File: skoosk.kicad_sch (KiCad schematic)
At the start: 90 parts, among them SW1 SW_Push, U1 ProMicro

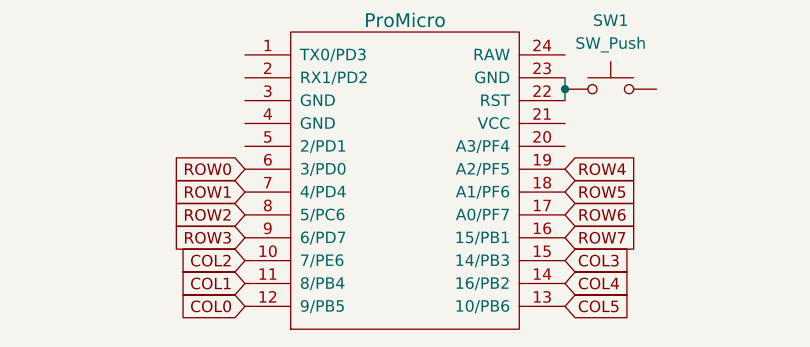
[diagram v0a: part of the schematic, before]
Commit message: saving before doing autorouting
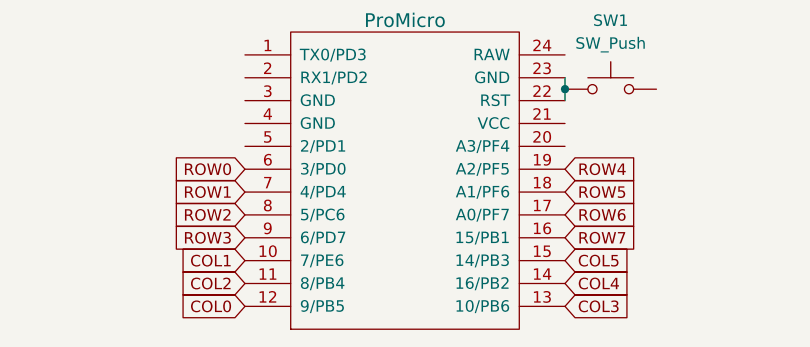
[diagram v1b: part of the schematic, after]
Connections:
- net COL1: now also U1.10 (7/PE6); no longer U1.11 (8/PB4)
- net COL2: now also U1.11 (8/PB4); no longer U1.10 (7/PE6)
- net COL3: now also U1.13 (10/PB6); no longer U1.15 (14/PB3)
- net COL5: now also U1.15 (14/PB3); no longer U1.13 (10/PB6)
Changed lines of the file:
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@@
     )
   )
-  (global_label "COL1" (shape input) (at 44.45 173.99 180) (fields_autoplaced)
+  (global_label "COL1" (shape input) (at 44.45 171.45 180) (fields_autoplaced)
     (effects (font (size 1.27 1.27)) (justify right))
-    (property "Intersheet References" "${INTERSHEET_REFS}" (id 0) (at 37.1988 174.0694 0)
+    (property "Intersheet References" "${INTERSHEET_REFS}" (id 0) (at 37.1988 171.5294 0)
       (effects (font (size 1.27 1.27)) (justify right) hide)
     )
@@
     )
   )
-  (global_label "COL5" (shape input) (at 80.01 176.53 0) (fields_autoplaced)
+  (global_label "COL5" (shape input) (at 80.01 171.45 0) (fields_autoplaced)
     (effects (font (size 1.27 1.27)) (justify left))
-    (property "Intersheet References" "${INTERSHEET_REFS}" (id 0) (at 87.2612 176.4506 0)
+    (property "Intersheet References" "${INTERSHEET_REFS}" (id 0) (at 87.2612 171.3706 0)
       (effects (font (size 1.27 1.27)) (justify left) hide)
     )
@@
     )
   )
-  (global_label "COL3" (shape input) (at 80.01 171.45 0) (fields_autoplaced)
+  (global_label "COL3" (shape input) (at 80.01 176.53 0) (fields_autoplaced)
     (effects (font (size 1.27 1.27)) (justify left))
-    (property "Intersheet References" "${INTERSHEET_REFS}" (id 0) (at 87.2612 171.3706 0)
+    (property "Intersheet References" "${INTERSHEET_REFS}" (id 0) (at 87.2612 176.4506 0)
       (effects (font (size 1.27 1.27)) (justify left) hide)
     )
@@
     )
   )
-  (global_label "COL2" (shape input) (at 44.45 171.45 180) (fields_autoplaced)
+  (global_label "COL2" (shape input) (at 44.45 173.99 180) (fields_autoplaced)
     (effects (font (size 1.27 1.27)) (justify right))
-    (property "Intersheet References" "${INTERSHEET_REFS}" (id 0) (at 37.1988 171.5294 0)
+    (property "Intersheet References" "${INTERSHEET_REFS}" (id 0) (at 37.1988 174.0694 0)
       (effects (font (size 1.27 1.27)) (justify right) hide)
     )
